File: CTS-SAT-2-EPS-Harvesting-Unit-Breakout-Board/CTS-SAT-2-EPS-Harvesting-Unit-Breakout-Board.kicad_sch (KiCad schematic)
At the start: 9 parts, among them J1 Conn_01x02_Pin, U1 MAX9922EUB+T

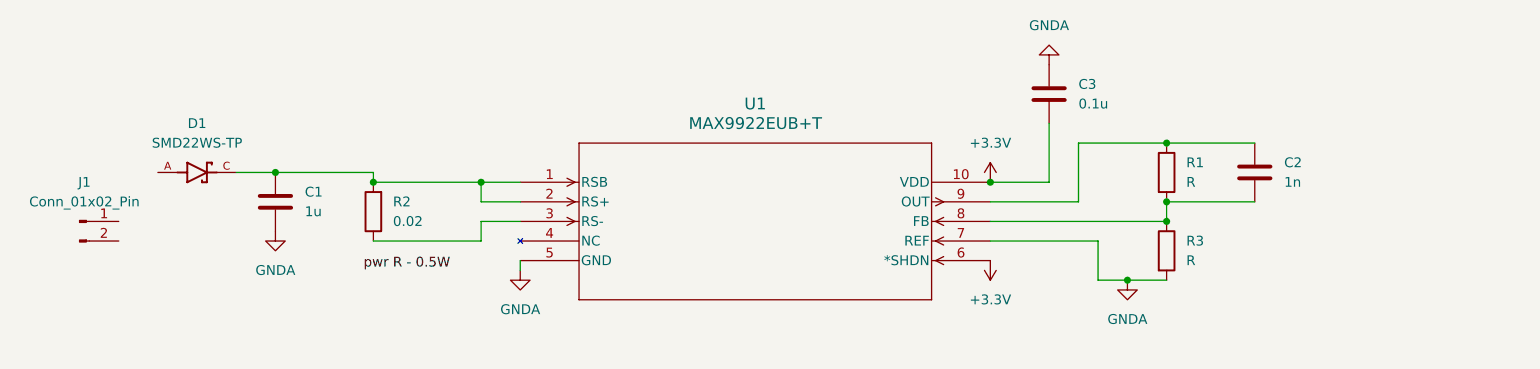
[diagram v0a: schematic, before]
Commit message: update
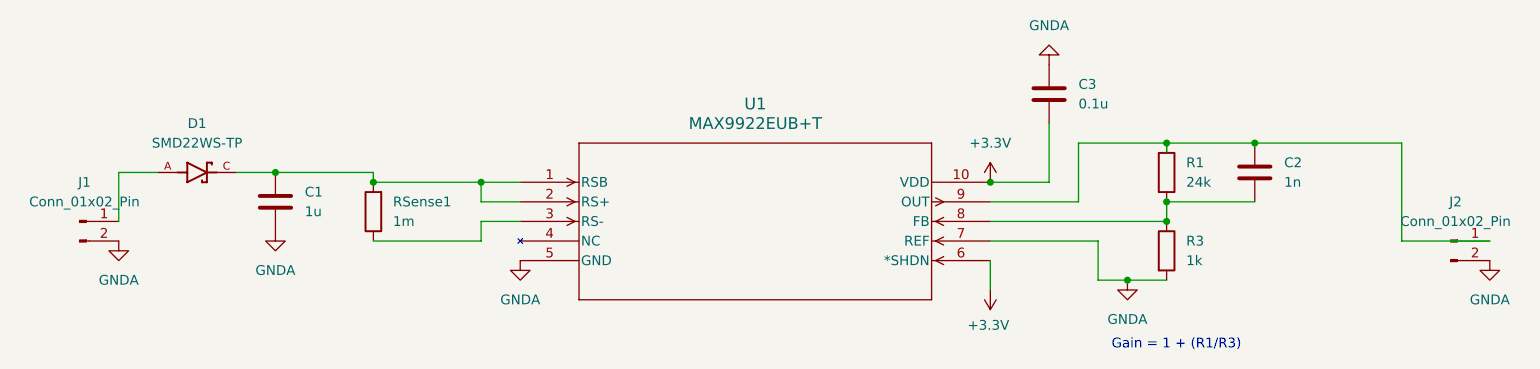
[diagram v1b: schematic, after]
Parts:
- added J2: Conn_01x02_Pin, Connector_PinHeader_2.54mm:PinHeader_1x02_P2.54mm_Vertical, symbol Connector:Conn_01x02_Pin
- R1: value R -> 24k
- R3: value R -> 1k
- RSense1: renamed from R2; value 0.02 -> 1m
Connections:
- net GNDA: now also J1.2 (Pin_2), J2.2 (Pin_2)
- net at D1.A: now also J1.1 (Pin_1)
- net at C2.1, R1.1, U1.9 (OUT): now also J2.1 (Pin_1)
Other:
- note added: "Gain = 1 + (R1/R3)"
